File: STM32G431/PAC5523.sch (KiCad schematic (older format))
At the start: 81 parts, among them J1 W, J2 U, J3 V, U1 STM32G431CBUx, U10 MIC4605, U12 AMS1117-3.3, U4 XL7015, U6 MIC4605, U7 MIC4605, Y1 8Mhz

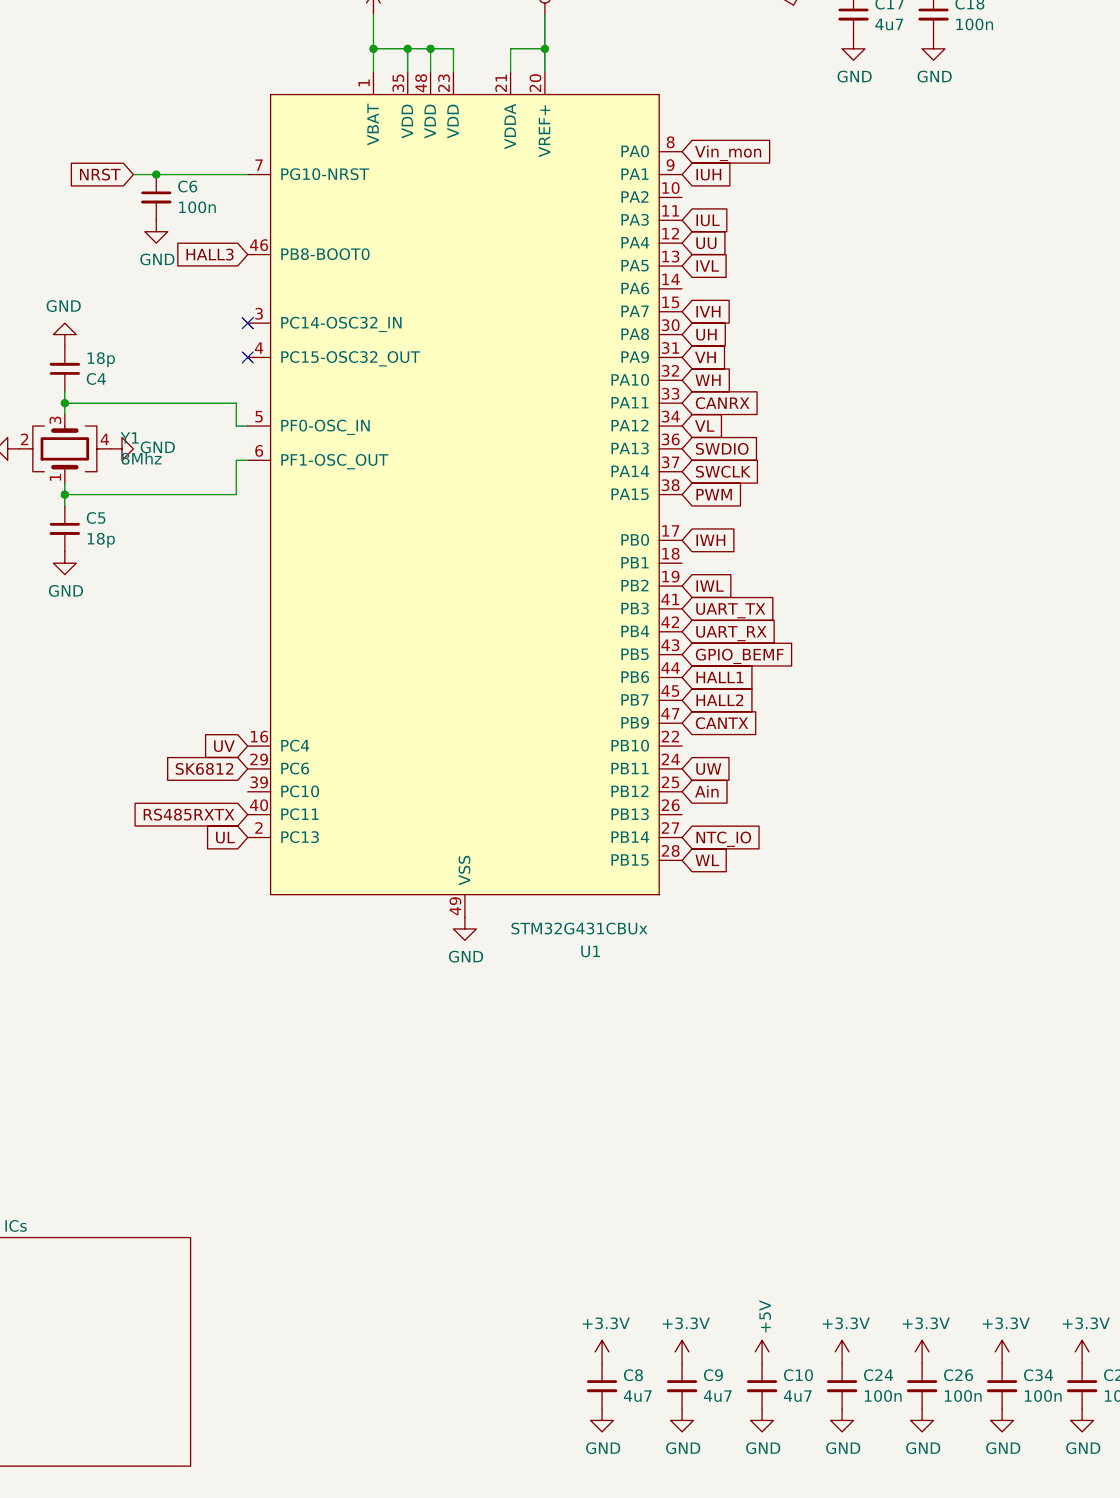
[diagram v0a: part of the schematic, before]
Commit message: updated files
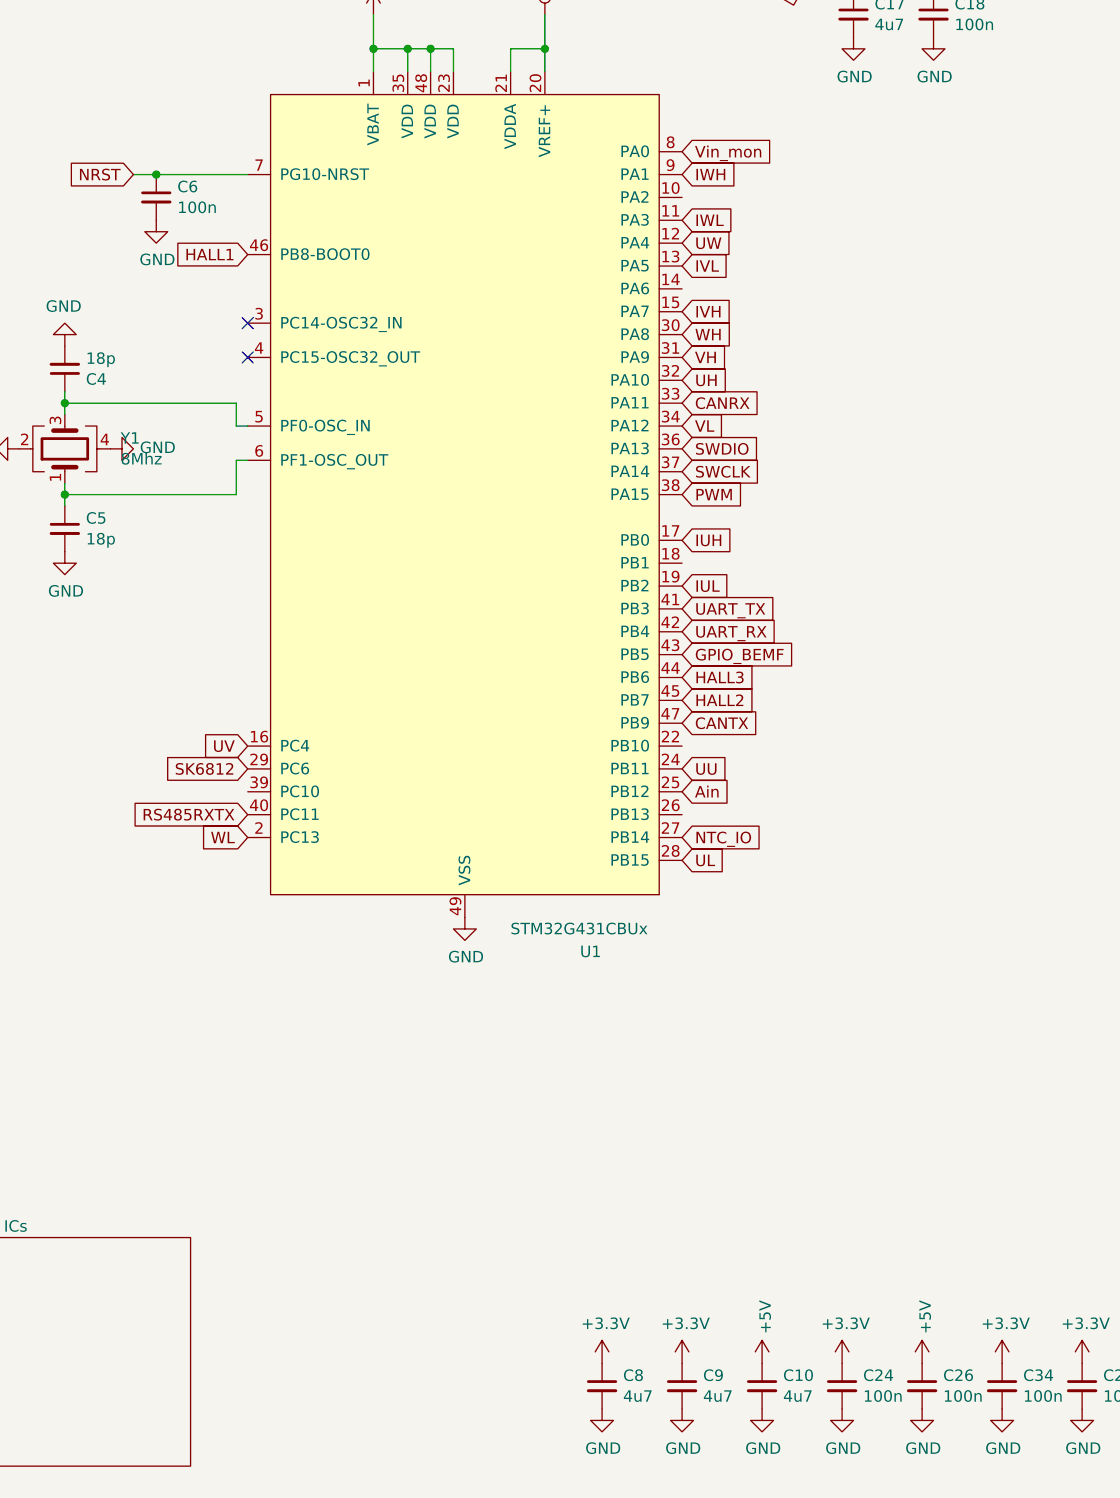
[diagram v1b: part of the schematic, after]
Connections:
- net +3V3: no longer C26.1
- net +5V: now also C26.1
- net HALL1: now also U1.46 (PB8-BOOT0); no longer U1.44 (PB6)
- net HALL3: now also U1.44 (PB6); no longer U1.46 (PB8-BOOT0)
- net IUH: now also U1.17 (PB0); no longer U1.9 (PA1)
- net IUL: now also U1.19 (PB2); no longer U1.11 (PA3)
- net IWH: now also U1.9 (PA1); no longer U1.17 (PB0)
- net IWL: now also U1.11 (PA3); no longer U1.19 (PB2)
- net UH: now also U1.32 (PA10); no longer U1.30 (PA8)
- net UL: now also U1.28 (PB15); no longer U1.2 (PC13)
- net UU: now also U1.24 (PB11); no longer U1.12 (PA4)
- net UW: now also U1.12 (PA4); no longer U1.24 (PB11)
- net WH: now also U1.30 (PA8); no longer U1.32 (PA10)
- net WL: now also U1.2 (PC13); no longer U1.28 (PB15)
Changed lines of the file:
@@
 Wire Wire Line
 	9200 6100 9200 6050
-Text GLabel 4600 4050 2    50   Input ~ 0
+Text GLabel 2700 2200 0    50   Input ~ 0
 HALL1
 Text GLabel 4600 4150 2    50   Input ~ 0
 HALL2
-Text GLabel 4600 3650 2    50   Input ~ 0
-IWL
-Text GLabel 4600 3450 2    50   Input ~ 0
-IWH
 Text GLabel 4600 2250 2    50   Input ~ 0
 IVL
 Text GLabel 4600 2450 2    50   Input ~ 0
 IVH
-Text GLabel 4600 2050 2    50   Input ~ 0
-IUL
-Text GLabel 4600 1850 2    50   Input ~ 0
-IUH
 $Comp
 L Connector:Conn_01x06_Male J2
@@
 Text GLabel 9650 1400 1    50   Input ~ 0
 U
-Text GLabel 4600 2150 2    50   Input ~ 0
-UU
 Text GLabel 2700 4350 0    50   Input ~ 0
 UV
-Text GLabel 4600 4450 2    50   Input ~ 0
-UW
 $Comp
 L Device:C_Small C34
@@
 Text GLabel 2200 1850 0    50   Input ~ 0
 NRST
-Text GLabel 2700 2200 0    50   Input ~ 0
+Text GLabel 4600 4050 2    50   Input ~ 0
 HALL3
 NoConn ~ 2700 2500
@@
 Text GLabel 8500 5100 0    50   Input ~ 0
 WL
-Text GLabel 4600 2550 2    50   Input ~ 0
-UH
-Text GLabel 2700 4750 0    50   Input ~ 0
-UL
 Text GLabel 4600 2650 2    50   Input ~ 0
 VH
 Text GLabel 4600 2950 2    50   Input ~ 0
 VL
-Text GLabel 4600 2750 2    50   Input ~ 0
-WH
-Text GLabel 4600 4850 2    50   Input ~ 0
-WL
 Wire Wire Line
 	10300 5150 10300 5250
@@
 F 3 "" H 5300 7050 50  0001 C CNN
 	1    5300 7050
-	1    0    0    -1
-$EndComp
-$Comp
-L power:+3.3V #PWR0184
-U 1 1 5E77D38A
-P 5650 7050
-F 0 "#PWR0184" H 5650 6900 50  0001 C CNN
-F 1 "+3.3V" H 5665 7223 50  0000 C CNN
-F 2 "" H 5650 7050 50  0001 C CNN
-F 3 "" H 5650 7050 50  0001 C CNN
-	1    5650 7050
 	1    0    0    -1
 $EndComp
@@
 	10450 4900 10450 4950
 Connection ~ 10450 4950
+$Comp
+L power:+5V #PWR?
+U 1 1 5DFF82C4
+P 5650 7050
+AR Path="/5D5C3A79/5DFF82C4" Ref="#PWR?"  Part="1"
+AR Path="/5DFF82C4" Ref="#PWR0184"  Part="1"
+F 0 "#PWR0184" H 5650 6900 50  0001 C CNN
+F 1 "+5V" V 5665 7178 50  0000 L CNN
+F 2 "" H 5650 7050 50  0001 C CNN
+F 3 "" H 5650 7050 50  0001 C CNN
+	1    5650 7050
+	1    0    0    -1
+$EndComp
+Text GLabel 4600 2050 2    50   Input ~ 0
+IWL
+Text GLabel 4600 1850 2    50   Input ~ 0
+IWH
+Text GLabel 4600 2150 2    50   Input ~ 0
+UW
+Text GLabel 4600 2550 2    50   Input ~ 0
+WH
+Text GLabel 4600 2750 2    50   Input ~ 0
+UH
+Text GLabel 4600 3450 2    50   Input ~ 0
+IUH
+Text GLabel 4600 3650 2    50   Input ~ 0
+IUL
+Text GLabel 4600 4450 2    50   Input ~ 0
+UU
+Text GLabel 4600 4850 2    50   Input ~ 0
+UL
+Text GLabel 2700 4750 0    50   Input ~ 0
+WL
 $EndSCHEMATC
